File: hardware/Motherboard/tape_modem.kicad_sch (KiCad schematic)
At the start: 1 part, among them U66 74LS273

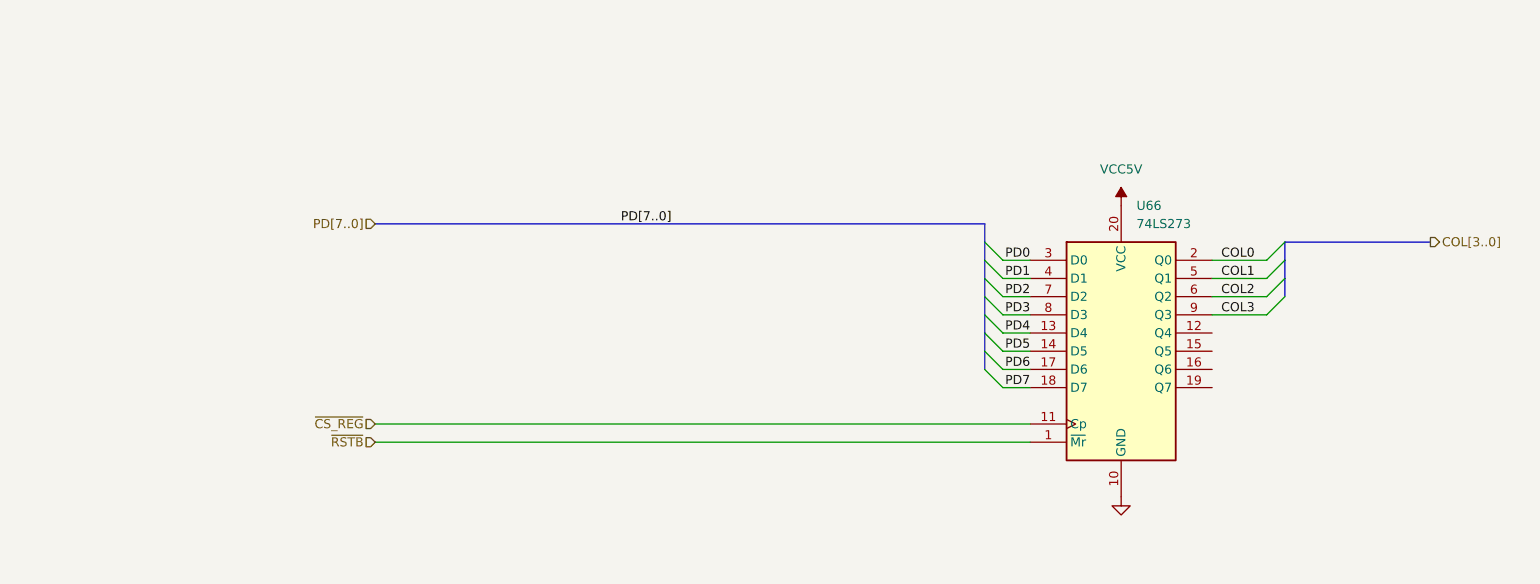
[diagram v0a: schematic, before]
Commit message: wip
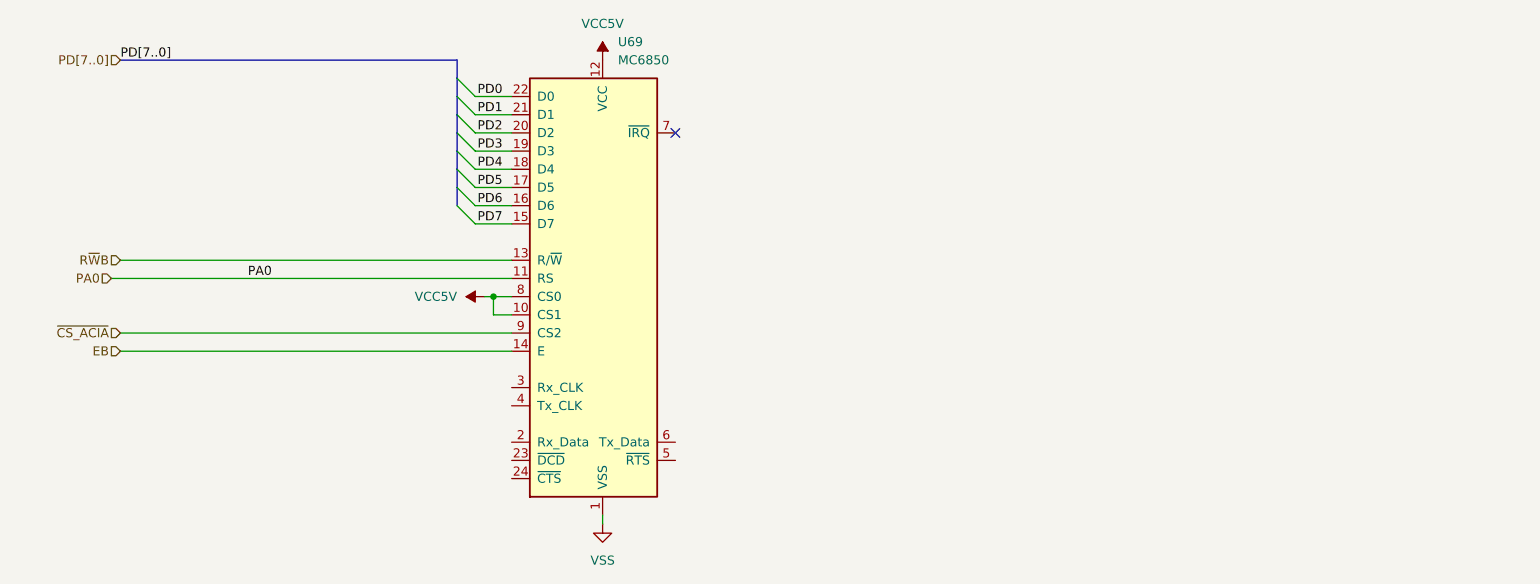
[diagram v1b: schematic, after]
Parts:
- removed U66: 74LS273, symbol 74xx:74LS273
- added U69: MC6850, Package_DIP:DIP-24_W15.24mm, symbol Interface_UART:MC6850
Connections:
- net PD0: now also U69.22 (D0)
- net PD1: now also U69.21 (D1)
- net PD2: now also U69.20 (D2)
- net PD3: now also U69.19 (D3)
- net PD4: now also U69.18 (D4)
- net PD5: now also U69.17 (D5)
- net PD6: now also U69.16 (D6)
- net PD7: now also U69.15 (D7)
- net VCC5V: now also U69.10 (CS1), U69.12 (VCC), U69.8 (CS0)
- net VSS: now also U69.1 (VSS)
- new net EB: U69.14 (E)
- new net PA0: U69.11 (RS)
- new net R~{W}B: U69.13 (R/~{W})
- new net ~{CS_ACIA}: U69.9 (CS2)
- no-connect marks 0 -> 1
